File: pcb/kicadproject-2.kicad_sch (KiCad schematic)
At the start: 9 parts, among them SW1 SW_Push, SW2 SW_Push, SW3 SW_Push, SW4 SW_Push, SW5 SW_Push, SW6 SW_Push, SW7 RotaryEncoder_Switch, U1 XIAO-RP2040-DIP, U2 OLED_0.91_128x32

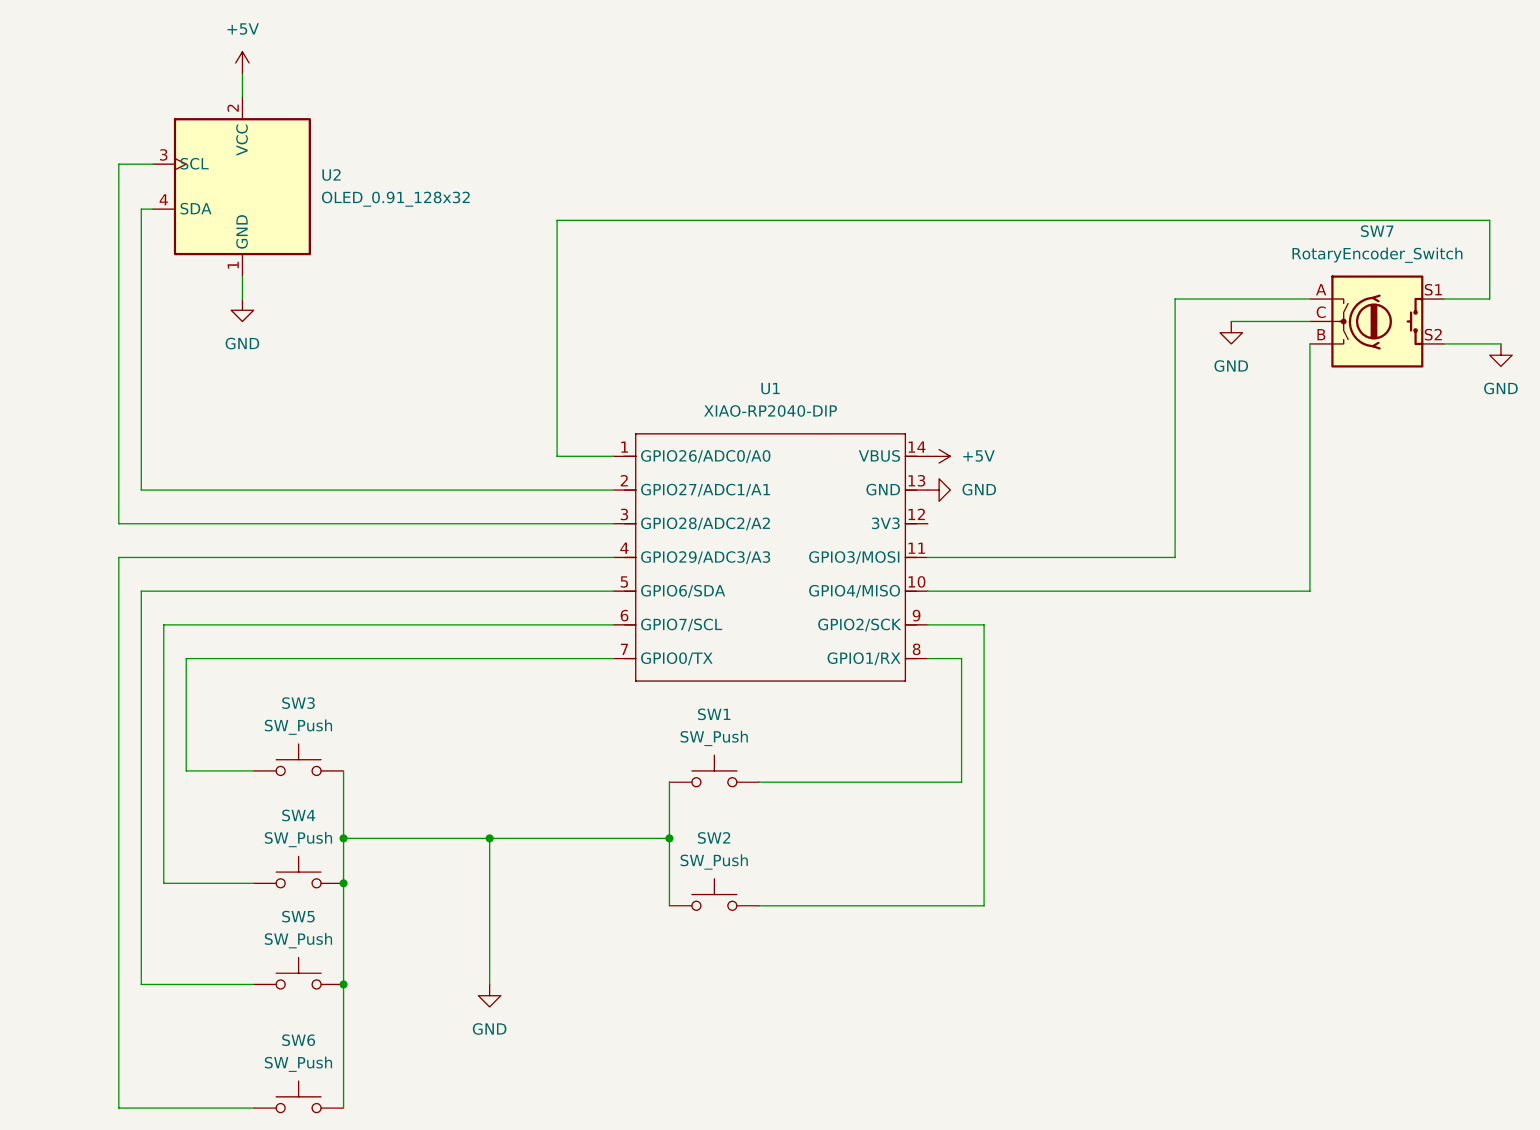
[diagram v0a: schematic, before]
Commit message: fixedpcb
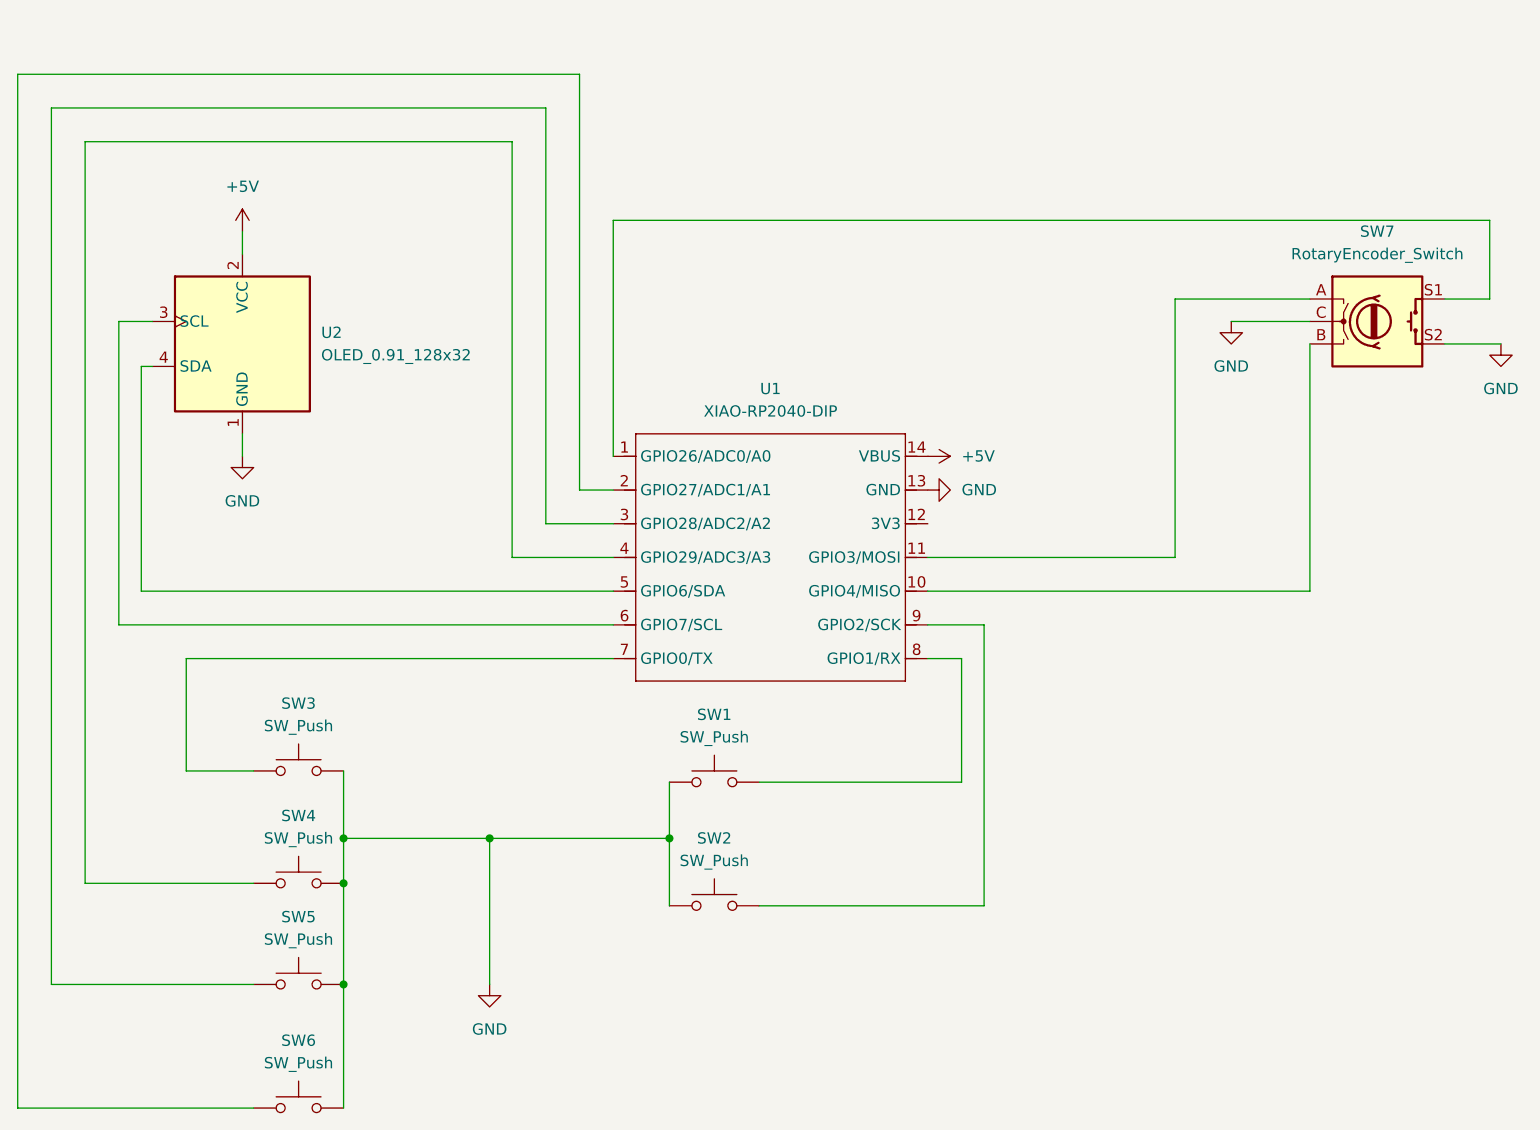
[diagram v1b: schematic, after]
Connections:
- net at SW5.1: now also U1.3 (GPIO28/ADC2/A2); no longer U1.5 (GPIO6/SDA)
- net at U1.2 (GPIO27/ADC1/A1): now also SW6.1; no longer U2.4 (SDA)
- net at U2.3 (SCL): now also U1.6 (GPIO7/SCL); no longer U1.3 (GPIO28/ADC2/A2)
- net at U1.4 (GPIO29/ADC3/A3): now also SW4.1; no longer SW6.1
- new net: U1.5 (GPIO6/SDA), U2.4 (SDA)
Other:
- moved on the sheet: U2
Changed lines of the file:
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@@
+	(wire
+		(pts
+			(xy 54.61 148.59) (xy 54.61 64.77)
+		)
+		(stroke
+			(width 0)
+			(type default)
+		)
+	)
 	(wire
 		(pts
@@
 	(wire
 		(pts
-			(xy 114.3 107.95) (xy 58.42 107.95)
-		)
-		(stroke
-			(width 0)
-			(type default)
-		)
-	)
-	(wire
-		(pts
 			(xy 153.67 123.19) (xy 153.67 137.16)
 		)
@@
 	(wire
 		(pts
-			(xy 72.39 57.15) (xy 72.39 59.69)
+			(xy 72.39 74.93) (xy 72.39 77.47)
 		)
 		(stroke
@@
 	(wire
 		(pts
-			(xy 107.95 100.33) (xy 114.3 100.33)
-		)
-		(stroke
-			(width 0)
-			(type default)
-		)
-	)
-	(wire
-		(pts
 			(xy 83.82 160.02) (xy 83.82 173.99)
 		)
@@
 	(wire
 		(pts
-			(xy 60.96 115.57) (xy 114.3 115.57)
-		)
-		(stroke
-			(width 0)
-			(type default)
-		)
-	)
-	(wire
-		(pts
-			(xy 73.66 160.02) (xy 60.96 160.02)
+			(xy 50.8 160.02) (xy 73.66 160.02)
+		)
+		(stroke
+			(width 0)
+			(type default)
+		)
+	)
+	(wire
+		(pts
+			(xy 102.87 111.76) (xy 114.3 111.76)
 		)
 		(stroke
@@
 	(wire
 		(pts
+			(xy 58.42 85.09) (xy 58.42 119.38)
+		)
+		(stroke
+			(width 0)
+			(type default)
+		)
+	)
+	(wire
+		(pts
+			(xy 213.36 73.66) (xy 114.3 73.66)
+		)
+		(stroke
+			(width 0)
+			(type default)
+		)
+	)
+	(wire
+		(pts
 			(xy 83.82 143.51) (xy 83.82 148.59)
 		)
@@
 	(wire
 		(pts
-			(xy 62.23 72.39) (xy 60.96 72.39)
+			(xy 54.61 148.59) (xy 73.66 148.59)
+		)
+		(stroke
+			(width 0)
+			(type default)
+		)
+	)
+	(wire
+		(pts
+			(xy 62.23 90.17) (xy 60.96 90.17)
 		)
 		(stroke
@@
 	(wire
 		(pts
+			(xy 50.8 60.96) (xy 50.8 160.02)
+		)
+		(stroke
+			(width 0)
+			(type default)
+		)
+	)
+	(wire
+		(pts
+			(xy 54.61 64.77) (xy 102.87 64.77)
+		)
+		(stroke
+			(width 0)
+			(type default)
+		)
+	)
+	(wire
+		(pts
 			(xy 100.33 143.51) (xy 120.65 143.51)
 		)
@@
 	(wire
 		(pts
-			(xy 63.5 148.59) (xy 63.5 119.38)
-		)
-		(stroke
-			(width 0)
-			(type default)
-		)
-	)
-	(wire
-		(pts
 			(xy 83.82 135.89) (xy 83.82 143.51)
 		)
@@
 	(wire
 		(pts
-			(xy 72.39 82.55) (xy 72.39 80.01)
+			(xy 72.39 100.33) (xy 72.39 97.79)
+		)
+		(stroke
+			(width 0)
+			(type default)
+		)
+	)
+	(wire
+		(pts
+			(xy 106.68 60.96) (xy 50.8 60.96)
 		)
 		(stroke
@@
 	(wire
 		(pts
-			(xy 63.5 119.38) (xy 114.3 119.38)
+			(xy 58.42 119.38) (xy 114.3 119.38)
 		)
 		(stroke
@@
 	(wire
 		(pts
-			(xy 60.96 104.14) (xy 114.3 104.14)
-		)
-		(stroke
-			(width 0)
-			(type default)
-		)
-	)
-	(wire
-		(pts
 			(xy 149.86 111.76) (xy 177.8 111.76)
 		)
@@
 	(wire
 		(pts
-			(xy 58.42 67.31) (xy 62.23 67.31)
-		)
-		(stroke
-			(width 0)
-			(type default)
-		)
-	)
-	(wire
-		(pts
-			(xy 114.3 111.76) (xy 58.42 111.76)
+			(xy 114.3 107.95) (xy 106.68 107.95)
+		)
+		(stroke
+			(width 0)
+			(type default)
+		)
+	)
+	(wire
+		(pts
+			(xy 46.99 173.99) (xy 73.66 173.99)
+		)
+		(stroke
+			(width 0)
+			(type default)
+		)
+	)
+	(wire
+		(pts
+			(xy 58.42 85.09) (xy 62.23 85.09)
+		)
+		(stroke
+			(width 0)
+			(type default)
+		)
+	)
+	(wire
+		(pts
+			(xy 60.96 115.57) (xy 60.96 90.17)
 		)
 		(stroke
@@
 	(wire
 		(pts
-			(xy 58.42 111.76) (xy 58.42 173.99)
+			(xy 114.3 73.66) (xy 114.3 100.33)
 		)
 		(stroke
@@
 	(wire
 		(pts
-			(xy 107.95 73.66) (xy 107.95 100.33)
+			(xy 110.49 57.15) (xy 110.49 104.14)
 		)
 		(stroke
@@
 	(wire
 		(pts
-			(xy 60.96 72.39) (xy 60.96 104.14)
-		)
-		(stroke
-			(width 0)
-			(type default)
-		)
-	)
-	(wire
-		(pts
-			(xy 60.96 160.02) (xy 60.96 115.57)
+			(xy 46.99 173.99) (xy 46.99 57.15)
+		)
+		(stroke
+			(width 0)
+			(type default)
+		)
+	)
+	(wire
+		(pts
+			(xy 102.87 64.77) (xy 102.87 111.76)
+		)
+		(stroke
+			(width 0)
+			(type default)
+		)
+	)
+	(wire
+		(pts
+			(xy 110.49 104.14) (xy 114.3 104.14)
+		)
+		(stroke
+			(width 0)
+			(type default)
+		)
+	)
+	(wire
+		(pts
+			(xy 46.99 57.15) (xy 110.49 57.15)
 		)
 		(stroke
@@
 	(wire
 		(pts
-			(xy 107.95 73.66) (xy 213.36 73.66)
-		)
-		(stroke
-			(width 0)
-			(type default)
-		)
-	)
-	(wire
-		(pts
-			(xy 58.42 107.95) (xy 58.42 67.31)
+			(xy 114.3 115.57) (xy 60.96 115.57)
 		)
 		(stroke
@@
 	(wire
 		(pts
-			(xy 73.66 148.59) (xy 63.5 148.59)
-		)
-		(stroke
-			(width 0)
-			(type default)
-		)
-	)
-	(wire
-		(pts
-			(xy 58.42 173.99) (xy 73.66 173.99)
+			(xy 106.68 107.95) (xy 106.68 60.96)
 		)
 		(stroke
@@
 	(symbol
 		(lib_id "power:GND")
-		(at 72.39 82.55 0)
+		(at 72.39 100.33 0)
 		(unit 1)
 		(exclude_from_sim no)
@@
 		(fields_autoplaced yes)
 		(property "Reference" "#PWR02"
-			(at 72.39 88.9 0)
+			(at 72.39 106.68 0)
 			(effects
 				(font
@@
 		)
 		(property "Value" "GND"
-			(at 72.39 87.63 0)
+			(at 72.39 105.41 0)
 			(effects
 				(font
@@
 		)
 		(property "Footprint" ""
-			(at 72.39 82.55 0)
+			(at 72.39 100.33 0)
 			(effects
 				(font
@@
 		)
 		(property "Datasheet" ""
-			(at 72.39 82.55 0)
+			(at 72.39 100.33 0)
 			(effects
 				(font
@@
 		)
 		(property "Description" "Power symbol creates a global label with name \"GND\" , ground"
-			(at 72.39 82.55 0)
+			(at 72.39 100.33 0)
 			(effects
 				(font
@@
 	(symbol
 		(lib_id "power:+5V")
-		(at 72.39 57.15 0)
+		(at 72.39 74.93 0)
 		(unit 1)
 		(exclude_from_sim no)
@@
 		(fields_autoplaced yes)
 		(property "Reference" "#PWR07"
-			(at 72.39 60.96 0)
+			(at 72.39 78.74 0)
 			(effects
 				(font
@@
 		)
 		(property "Value" "+5V"
-			(at 72.39 52.07 0)
+			(at 72.39 69.85 0)
 			(effects
 				(font
@@
 		)
 		(property "Footprint" ""
-			(at 72.39 57.15 0)
+			(at 72.39 74.93 0)
 			(effects
 				(font
@@
 		)
 		(property "Datasheet" ""
-			(at 72.39 57.15 0)
+			(at 72.39 74.93 0)
 			(effects
 				(font
@@
 		)
 		(property "Description" "Power symbol creates a global label with name \"+5V\""
-			(at 72.39 57.15 0)
+			(at 72.39 74.93 0)
 			(effects
 				(font
@@
 	(symbol
 		(lib_id "Hackclub Symbols:OLED_0.91_128x32")
-		(at 72.39 69.85 0)
+		(at 72.39 87.63 0)
 		(unit 1)
 		(exclude_from_sim no)
@@
 		(fields_autoplaced yes)
 		(property "Reference" "U2"
-			(at 81.28 68.5799 0)
+			(at 81.28 86.3599 0)
 			(effects
 				(font
@@
 		)
 		(property "Value" "OLED_0.91_128x32"
-			(at 81.28 71.1199 0)
+			(at 81.28 88.8999 0)
 			(effects
 				(font
@@
 		)
 		(property "Footprint" "Hackclub Footprints:OLED_0.91_128x32"
-			(at 90.424 82.55 0)
+			(at 90.424 100.33 0)
 			(effects
 				(font
@@
 		)
 		(property "Datasheet" "https://www.buydisplay.com/download/manual/ER-OLEDM0.91-1_Datasheet.pdf"
-			(at 115.062 84.582 0)
+			(at 115.062 102.362 0)
 			(effects
 				(font
@@
 		)
 		(property "Description" "SSD1306 OLED module, 0.91 inch, 128x32, I2C"
-			(at 99.06 86.614 0)
-			(effects
-				(font
+			(at 99.06 104.394 0)
+			(effects
+				(font
